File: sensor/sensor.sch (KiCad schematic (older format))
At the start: 5 parts, among them T1 DS18B20, T2 DS18B20, U1 DHT22, U2 SSCDRNN015PASA5

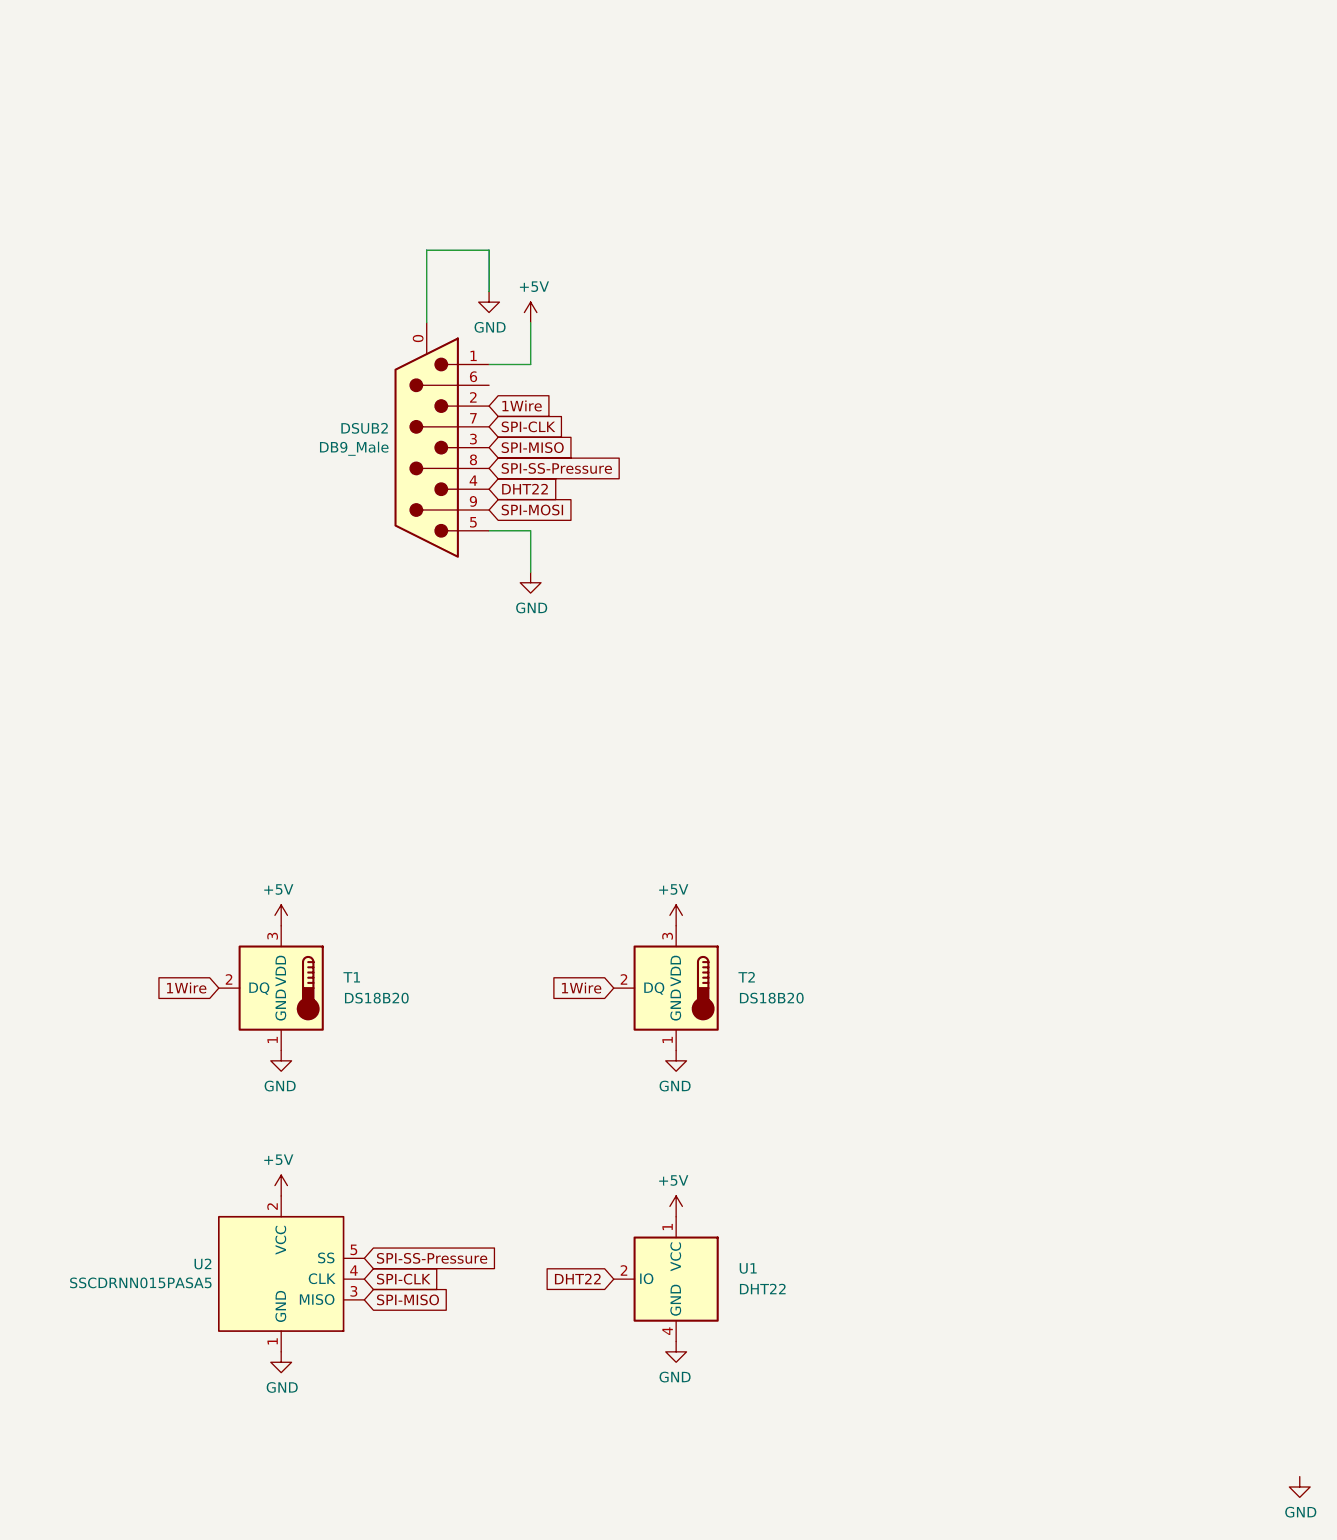
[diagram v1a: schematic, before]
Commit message: WIP sensor PCB
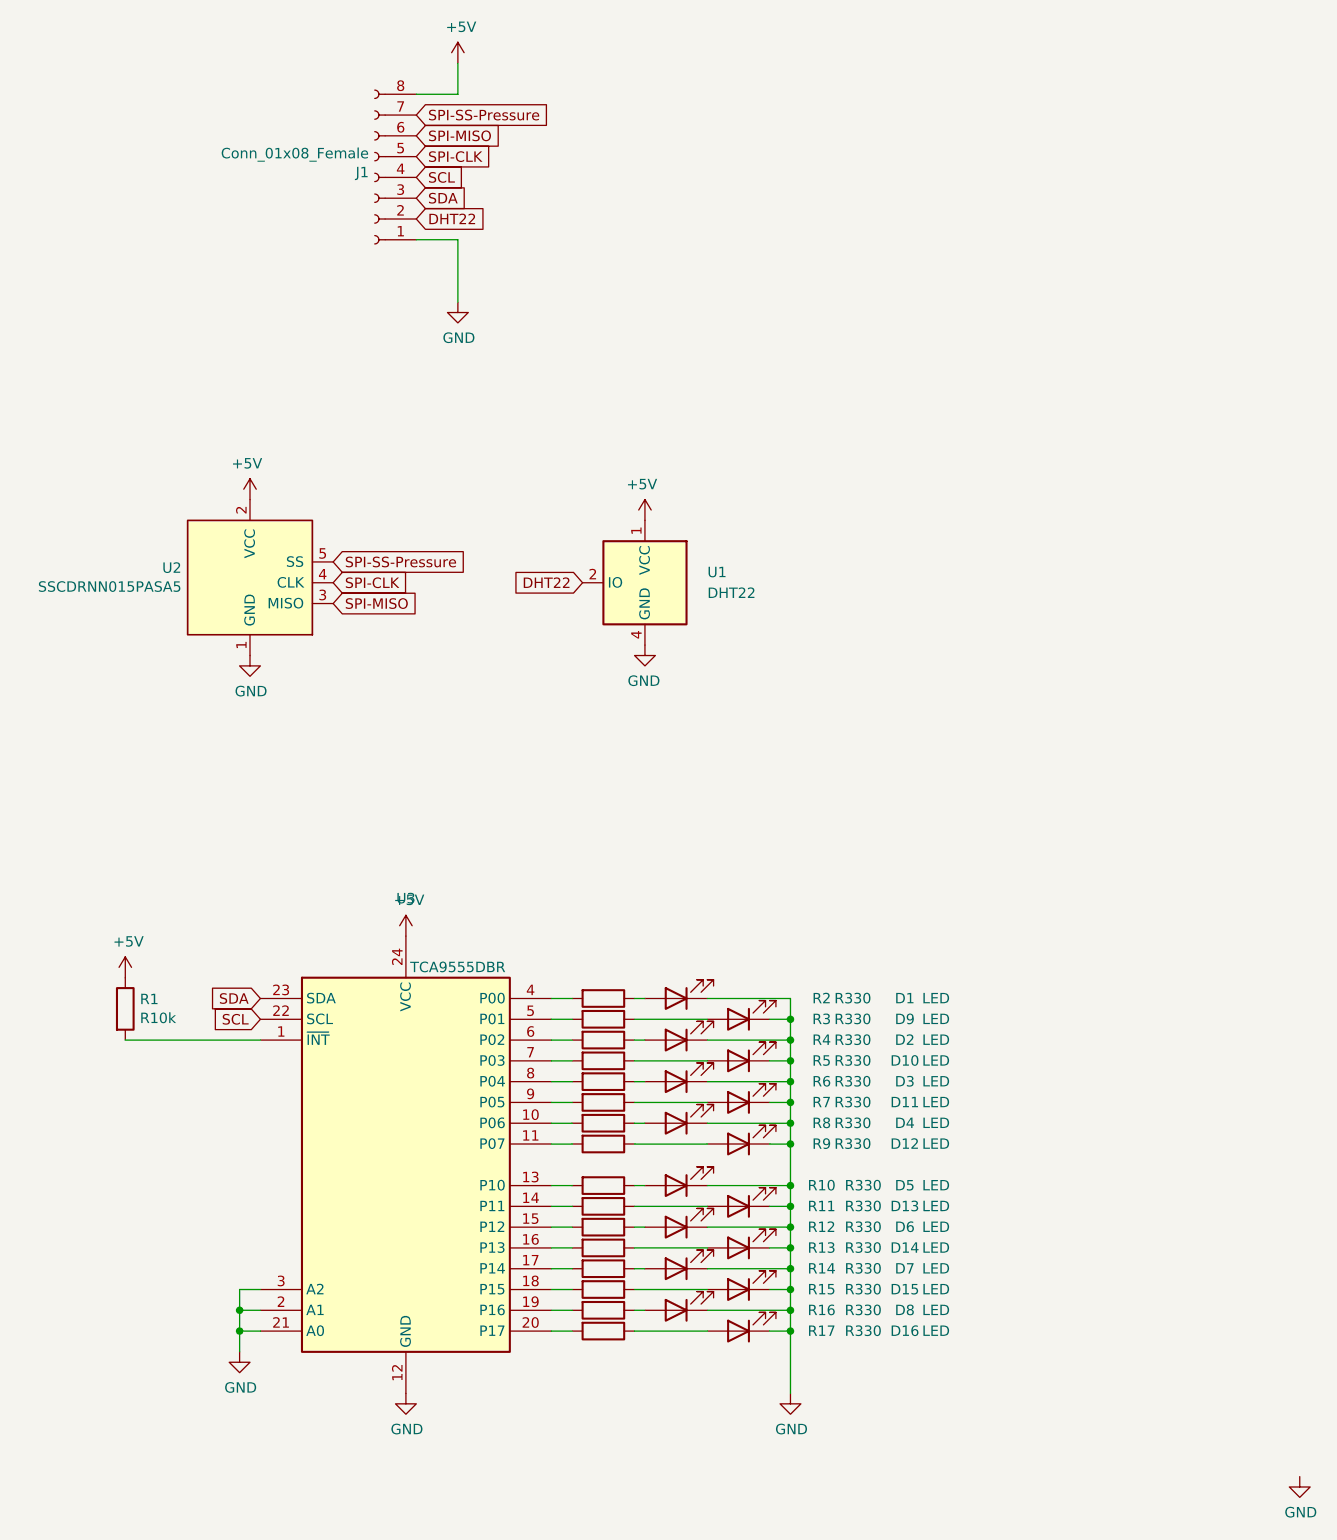
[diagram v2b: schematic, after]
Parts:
- removed DSUB2: DB9_Male, Connector_Dsub:DSUB-9_Male_Horizontal_P2.77x2.84mm_EdgePinOffset7.70mm_Housed_MountingHolesOffset9.12mm, symbol Connector:DB9_Male_MountingHoles
- removed T1, T2: DS18B20, Package_TO_SOT_THT:TO-92_Inline_Wide, symbol Sensor_Temperature:DS18B20
- added D1, D10, D11, D12, D13, D14, D15, D16, D2, D3, D4, D5, D6, D7, D8, D9: LED, LED_SMD:LED_0805_2012Metric_Pad1.15x1.40mm_HandSolder, symbol Device:LED
- added J1: Conn_01x08_Female, Stardust:691382040008, symbol Connector:Conn_01x08_Female
- added R1: R10k, Resistor_SMD:R_0603_1608Metric_Pad0.98x0.95mm_HandSolder, symbol Device:R
- added R10, R11, R12, R13, R14, R15, R16, R17, R2, R3, R4, R5, R6, R7, R8, R9: R330, Resistor_SMD:R_0603_1608Metric, symbol Device:R
- added U3: TCA9555DBR, Package_SO:SSOP-24_5.3x8.2mm_P0.65mm, symbol Interface_Expansion:TCA9555DBR
- U1: footprint Sensor:Aosong_DHT11_5.5x12.0_P2.54mm -> Stardust:DHT22_15.0x25.0_P2.54mm_Horizontal
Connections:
- net +5V: now also J1.8 (Pin_8), R1.1, U3.24 (VCC)
- net DHT22: now also J1.2 (Pin_2)
- net GND: now also D1.1 (K), D10.1 (K), D11.1 (K), D12.1 (K), D13.1 (K), D14.1 (K), D15.1 (K), D16.1 (K), D2.1 (K), D3.1 (K), D4.1 (K), D5.1 (K), D6.1 (K), D7.1 (K), D8.1 (K), D9.1 (K), J1.1 (Pin_1), U3.12 (GND), U3.2 (A1), U3.21 (A0), U3.3 (A2)
- net SPI-CLK: now also J1.5 (Pin_5)
- net SPI-MISO: now also J1.6 (Pin_6)
- net SPI-SS-Pressure: now also J1.7 (Pin_7)
- new net: D9.2 (A), R3.1
- new net: D2.2 (A), R4.1
- new net: R4.2, U3.6 (P02)
- new net: D10.2 (A), R5.1
- new net: R5.2, U3.7 (P03)
- new net: D3.2 (A), R6.1
- new net: R6.2, U3.8 (P04)
- new net: D11.2 (A), R7.1
- new net: R7.2, U3.9 (P05)
- new net: D4.2 (A), R8.1
- new net: R8.2, U3.10 (P06)
- new net: D12.2 (A), R9.1
- new net: R9.2, U3.11 (P07)
- new net: D5.2 (A), R10.1
- new net: R10.2, U3.13 (P10)
- new net: D13.2 (A), R11.1
- new net: R11.2, U3.14 (P11)
- new net: D6.2 (A), R12.1
- new net: R12.2, U3.15 (P12)
- new net: D14.2 (A), R13.1
- new net: R13.2, U3.16 (P13)
- new net: D7.2 (A), R14.1
- new net: R14.2, U3.17 (P14)
- new net: D15.2 (A), R15.1
- new net: R15.2, U3.18 (P15)
- new net: D8.2 (A), R16.1
- new net: R16.2, U3.19 (P16)
- new net: D16.2 (A), R17.1
- new net: R17.2, U3.20 (P17)
- new net: R1.2, U3.1 (~INT)
- new net: R2.2, U3.4 (P00)
- new net: R3.2, U3.5 (P01)
- new net: D1.2 (A), R2.1
- new net SCL: J1.4 (Pin_4), U3.22 (SCL)
- new net SDA: J1.3 (Pin_3), U3.23 (SDA)
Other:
- moved on the sheet: U1, U2

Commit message: WIP sensor PCB - delete files
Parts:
- U2: symbol sscdrnn015pasa5:SSCDRNN015PASA5 -> Stardust:SSCDRNN015PASA5
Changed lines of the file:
@@
 SPI-CLK
 $Comp
-L sscdrnn015pasa5:SSCDRNN015PASA5 U2
+L Stardust:SSCDRNN015PASA5 U2
 U 1 1 5EA36ED1
 P 2950 4650

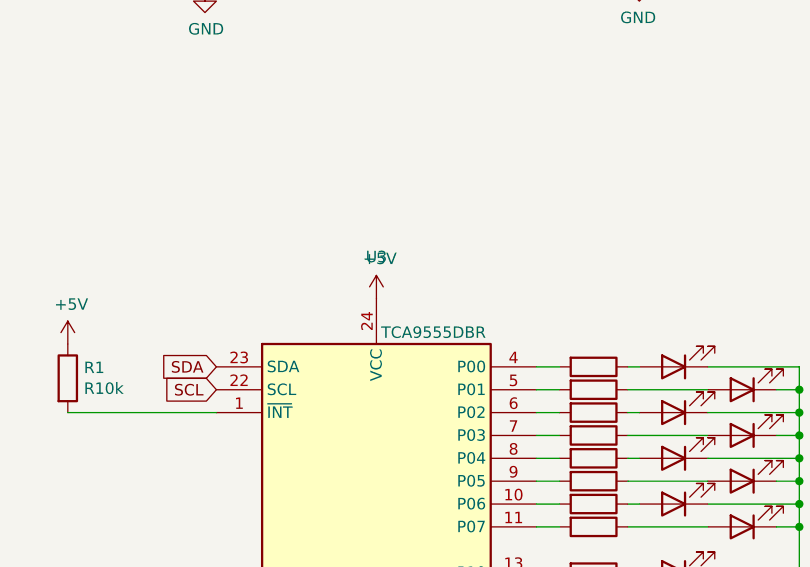
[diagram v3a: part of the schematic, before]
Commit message: WIP
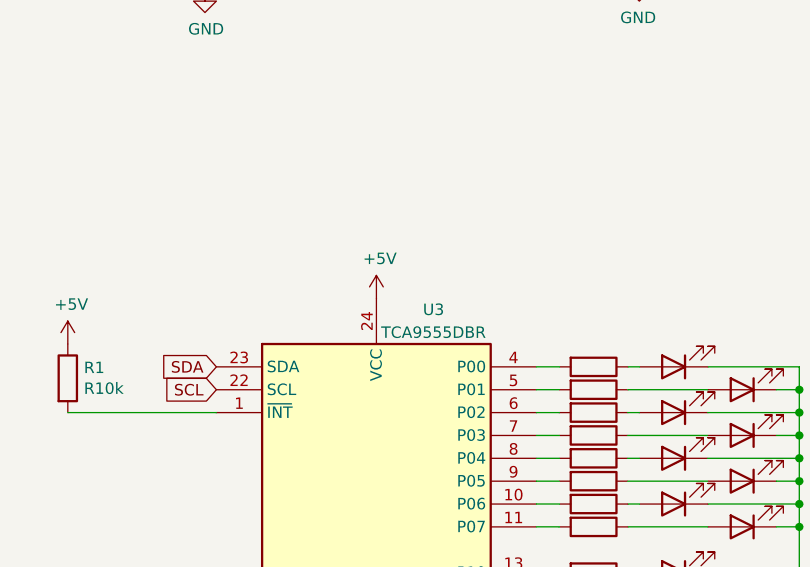
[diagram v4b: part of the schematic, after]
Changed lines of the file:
@@
 U 1 1 601916EE
 P 3700 6900
-F 0 "U3" H 3700 8181 50  0000 C CNN
+F 0 "U3" H 3950 7950 50  0000 C CNN
 F 1 "TCA9555DBR" H 3950 7850 50  0000 C CNN
 F 2 "Package_SO:SSOP-24_5.3x8.2mm_P0.65mm" H 4750 5900 50  0001 C CNN
